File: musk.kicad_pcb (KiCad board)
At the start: 2 copper layers, 104 x 106 mm, 104 parts, among them J1 debug-port, J10 Conn_01x06_Male, J2 USB_C_Receptacle_USB2.0, J3 Conn_01x06_Male, J4 Conn_01x06_Male, J5 Conn_01x06_Male, J6 Conn_01x06_Male, J7 Conn_01x06_Male, J8 Conn_01x06_Male, J9 Conn_01x06_Male, K1 diode-choc, K10 diode-choc, K11 diode-choc, K12 diode-choc, K13 diode-choc, K14 diode-choc, K15 diode-choc, K16 diode-choc, K17 diode-choc, K2 diode-choc, K3 diode-choc, K4 diode-choc, K5 diode-choc, K6 diode-choc, K7 diode-choc, K8 diode-choc, K9 diode-choc, Q1 BC807, SW1 SW_Push, SW2 RotaryEncoder, U1 MT25QL128ABA1ESE, U10 LM397, U2 ms88sf3-nrf52840, U3 LSM6DS3, U4 XC6220B331MR, U6 SRV05-4, U8 PMW3610, U9 MCP1804x-1802xMB

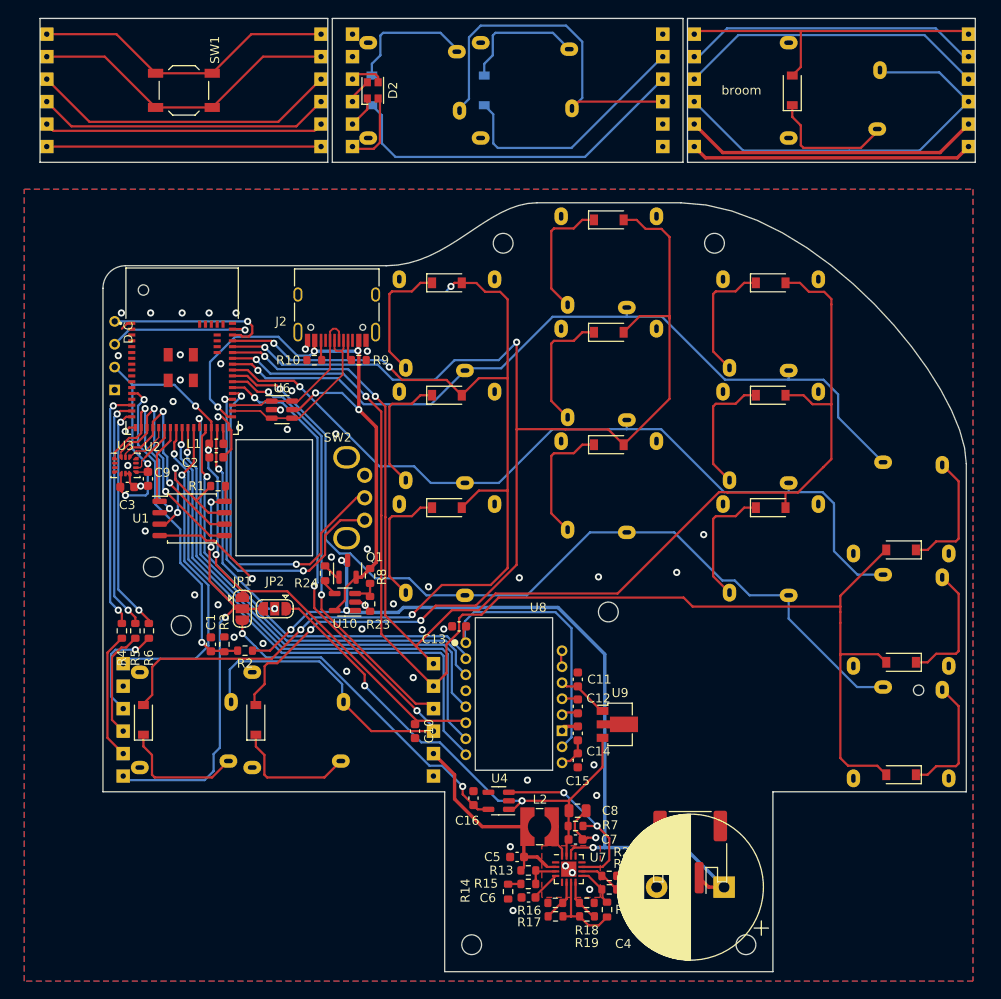
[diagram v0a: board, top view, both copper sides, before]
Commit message: swap bms and reg
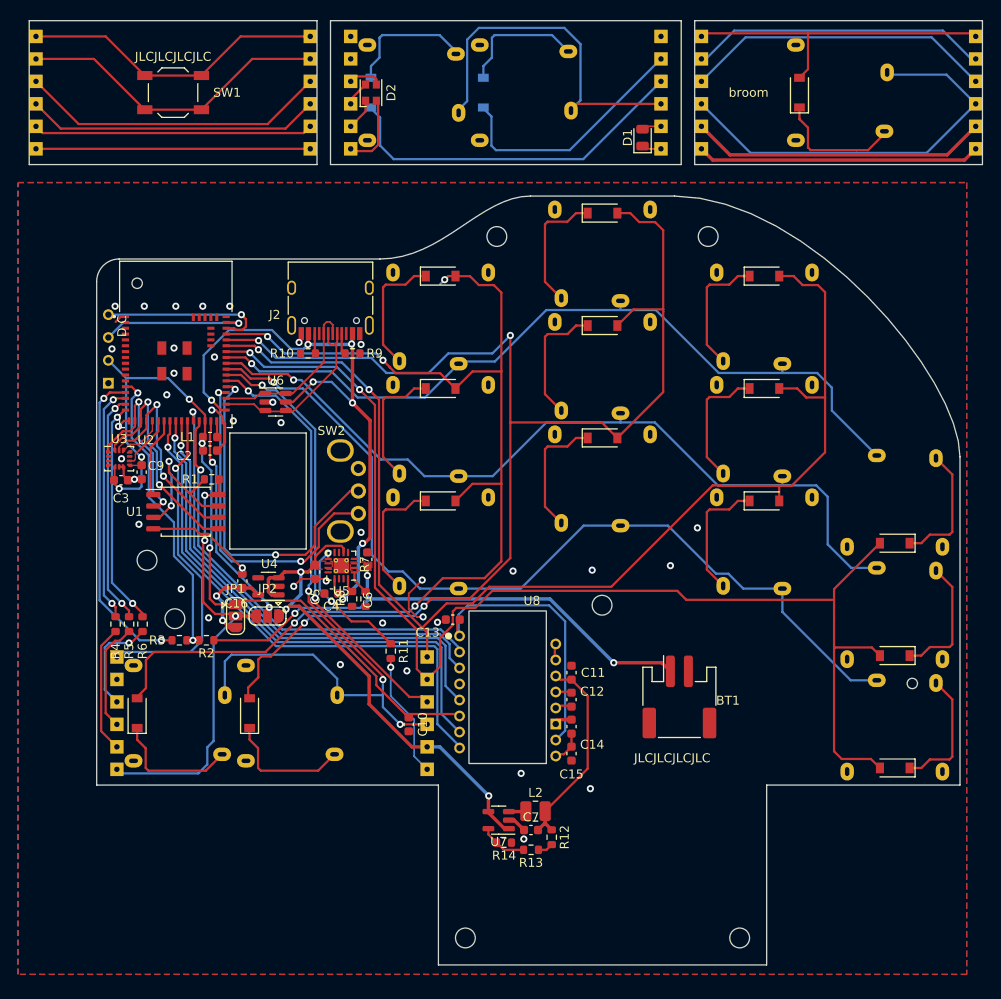
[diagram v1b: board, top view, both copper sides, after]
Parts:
- removed C1: 10nF, Capacitor_SMD:C_0603_1608Metric
- removed C8: 4.7uF, Capacitor_SMD:C_0805_2012Metric
- removed Q1: BC807, Package_TO_SOT_SMD:SOT-23
- removed R15: 5.9M, Resistor_SMD:R_0603_1608Metric
- removed R16, R17, R18, R19: 5.1M, Resistor_SMD:R_0603_1608Metric
- removed R20: 1M, Resistor_SMD:R_0603_1608Metric
- removed R21: 4.12M, Resistor_SMD:R_0603_1608Metric
- removed R22: 4.87M, Resistor_SMD:R_0603_1608Metric
- removed R23: 8.2k, Resistor_SMD:R_0603_1608Metric
- removed R24: ?, Resistor_SMD:R_0603_1608Metric
- removed U10: LM397, Package_TO_SOT_SMD:SOT-23-5
- removed U9: MCP1804x-1802xMB, Package_TO_SOT_SMD:SOT-89-3
- added D1: RED, LED_SMD:LED_0805_2012Metric, F.Cu at (125.2, 26.0)
- added R11: 1k, Resistor_SMD:R_0603_1608Metric, F.Cu at (97.2, 83.1)
- added R12: 100k, Resistor_SMD:R_0603_1608Metric, F.Cu at (115.1, 103.8)
- added U5: BQ24072, Package_DFN_QFN:VQFN-16-1EP_3x3mm_P0.5mm_EP1.68x1.68mm_ThermalVias, F.Cu at (91.7, 73.6)
- C12: value 100uF -> 100nF
- C4: value Li Cap -> 4.7uF; footprint Capacitor_THT:CP_Radial_D16.0mm_P7.50mm -> Capacitor_SMD:C_0603_1608Metric
- C6: value 10nF -> 4.7uF
- C7: value 0.1uF -> 10uF
- L2: value 22uH -> 2.2uH; footprint Inductor_SMD:L_Wuerth_WE-TPC-3816 -> Inductor_SMD:L_1008_2520Metric
- R13: value 4.12M -> 100k
- R14: value 10M -> 100k
- R2, R3: value 5.1M -> 100k
- R7: value 1M -> 10k
- R8: value 2.8k -> 10k
- U1: value MT25QL128ABA1ESE -> W25Q128
- U7: value ~ -> TLV62568DBV; footprint Package_DFN_QFN:QFN-16-1EP_3x3mm_P0.5mm_EP1.7x1.7mm -> Package_TO_SOT_SMD:SOT-23-5
- moved C4 51.5 mm to (90.6, 76.7)
- moved C6 41.6 mm to (94.6, 72.9), turned to 90 degrees
- moved C5 38.8 mm to (88.8, 74.3), turned to 90 degrees
- moved C16 35.3 mm to (80.7, 75.3)
- moved U4 35.0 mm to (83.6, 75.9)
- moved R7 34.4 mm to (94.4, 77.3), turned to -90 degrees
- moved BT1 17.3 mm to (129.3, 88.2), turned to 0 degrees
- moved U7 9.52 mm to (109.2, 101.9), turned to 180 degrees
- moved R14 5.47 mm to (109.8, 104.4), turned to 180 degrees
- moved C7 5.06 mm to (112.8, 103.0), turned to 0 degrees
- moved R3 5.02 mm to (73.7, 81.9), turned to 180 degrees
- moved R2 4.45 mm to (76.7, 81.9)
- moved R8 3.24 mm to (92.9, 77.3), turned to -90 degrees
- moved R13 2.31 mm to (112.8, 105.2), turned to 180 degrees
- moved L2 1.78 mm to (113.3, 100.9), turned to 0 degrees
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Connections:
- C4 pad 1: BAT -> VBUS
- C5 pad 2: SOLAR -> VDDH_OUT
- C6 pad 1: GND -> BAT
- C6 pad 2: Net-(C6-Pad2) -> GND
- C7 pad 2: SOLAR_OUT -> +1V8
- J8 pad 5: unconnected-(J8-Pad5) -> VDDH_OUT
- J8 pad 6: unconnected-(J8-Pad6) -> Net-(J8-Pad6)
- J9 pad 1: unconnected-(J9-Pad1) -> Net-(D1-Pad1)
- J9 pad 2: unconnected-(J9-Pad2) -> Net-(D1-Pad2)
- JP2 pad 1: SOLAR_OUT -> VDDH_OUT
- L2 pad 1: SOLAR -> Net-(L2-Pad1)
- L2 pad 2: Net-(L2-Pad2) -> +1V8
- R13 pad 1: SOLAR -> Net-(R12-Pad2)
- R14 pad 2: Net-(R14-Pad2) -> Net-(R13-Pad2)
- R3 pad 2: GND -> BAT_MEAS_EN
- R7 pad 2: SOLAR_OUT -> GND
- R8 pad 2: VBUS -> GND
- U2 pad 14: unconnected-(U2-Pad14) -> BAT_MEAS_EN
- U4 pad 1: SOLAR_OUT -> VDDH_OUT
- U4 pad 3: Net-(R7-Pad1) -> VDDH_OUT
- U7 pad 1: GND -> VDDH_OUT
- U7 pad 2: SOLAR -> GND
- U7 pad 3: Net-(R13-Pad2) -> Net-(L2-Pad1)
- U7 pad 4: Net-(C6-Pad2) -> VDDH_OUT
- U7 pad 5: GND -> Net-(R13-Pad2)
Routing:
- net SOLAR_OUT: track 58.6 -> 0.00 mm, vias 2 -> 0
- net VDDH_OUT: track 0.00 -> 57.9 mm, vias 0 -> 3
- net BAT_MEAS_EN: track 0.00 -> 35.2 mm, vias 0 -> 2
- net BAT: track 94.8 -> 59.8 mm, vias 4 -> 3
- net 3V3_LDO: track 37.4 -> 10.1 mm
- net SOLAR: track 24.0 -> 0.00 mm
- net Net-(R7-Pad1): track 20.6 -> 2.64 mm, vias 2 -> 0
- net +1V8: track 6.25 -> 23.2 mm
- net ~{CHG}: track 0.00 -> 15.5 mm, vias 0 -> 2
- net Net-(J8-Pad6): track 0.00 -> 14.0 mm, vias 0 -> 1
- net Net-(R17-Pad2): track 9.48 -> 0.00 mm
- net Net-(R18-Pad2): track 4.58 -> 0.00 mm
- net Net-(R16-Pad2): track 4.58 -> 0.00 mm
- net Net-(R21-Pad2): track 4.54 -> 0.00 mm
- net Net-(R20-Pad1): track 4.39 -> 0.00 mm
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- added copper zone on F.Cu, net BAT
- added copper zone on F.Cu, net VDDH_OUT
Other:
- board size 104 x 106 mm -> 106 x 105 mm
- board text added: "JLCJLCJLCJLC"
